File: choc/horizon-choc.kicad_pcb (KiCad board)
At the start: 2 copper layers, 252 x 68 mm, 63 parts, among them SW1 SW_Push, SW10 SW_Push, SW11 SW_Push, SW12 SW_Push, SW13 SW_Push, SW14 SW_Push, SW15 SW_Push, SW16 SW_Push, SW17 SW_Push, SW18 SW_Push, SW19 SW_Push, SW2 SW_Push, SW20 SW_Push, SW21 SW_Push, SW22 SW_Push, SW23 SW_Push, SW24 SW_Push, SW25 SW_Push, SW26 SW_Push, SW27 SW_Push, SW28 SW_Push, SW29 SW_Push, SW3 SW_Push, SW30 SW_Push, SW31 SW_Push, SW32 SW_Push, SW33 SW_Push, SW34 SW_Push, SW35 SW_Push, SW36 SW_Push, SW37 SW_Push, SW38 SW_Push, SW39 SW_Push, SW4 SW_Push, SW40 SW_Push, SW41 SW_Push, SW42 SW_Push, SW43 SW_Push, SW44 SW_Push, SW45 SW_Push, SW46 SW_Push, SW47 SW_Push, SW48 SW_Push, SW49 SW_Push, SW5 SW_Push, SW50 SW_Push, SW51 SW_Push, SW52 SW_Push, SW6 SW_Push, SW7 SW_Push, SW8 SW_Push, SW9 SW_Push, U1 PRO-MICRO

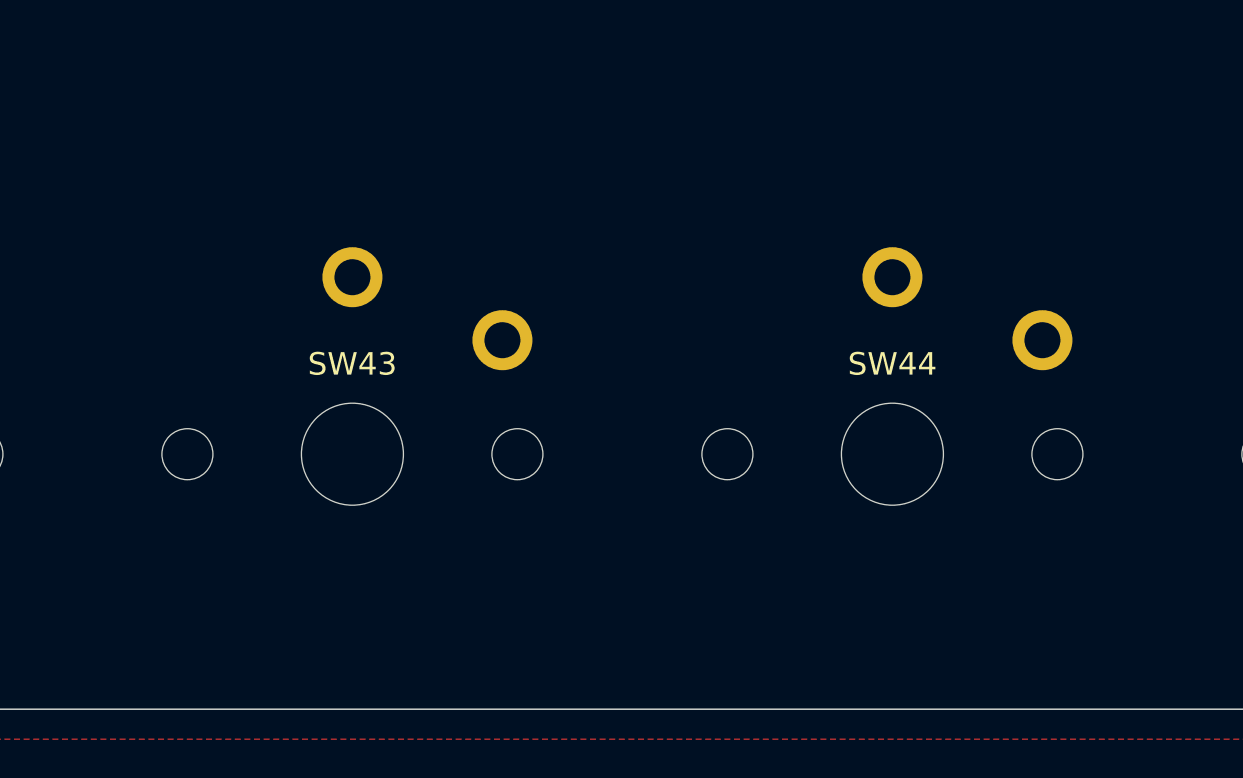
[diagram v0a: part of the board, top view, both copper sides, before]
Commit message: updated pcb
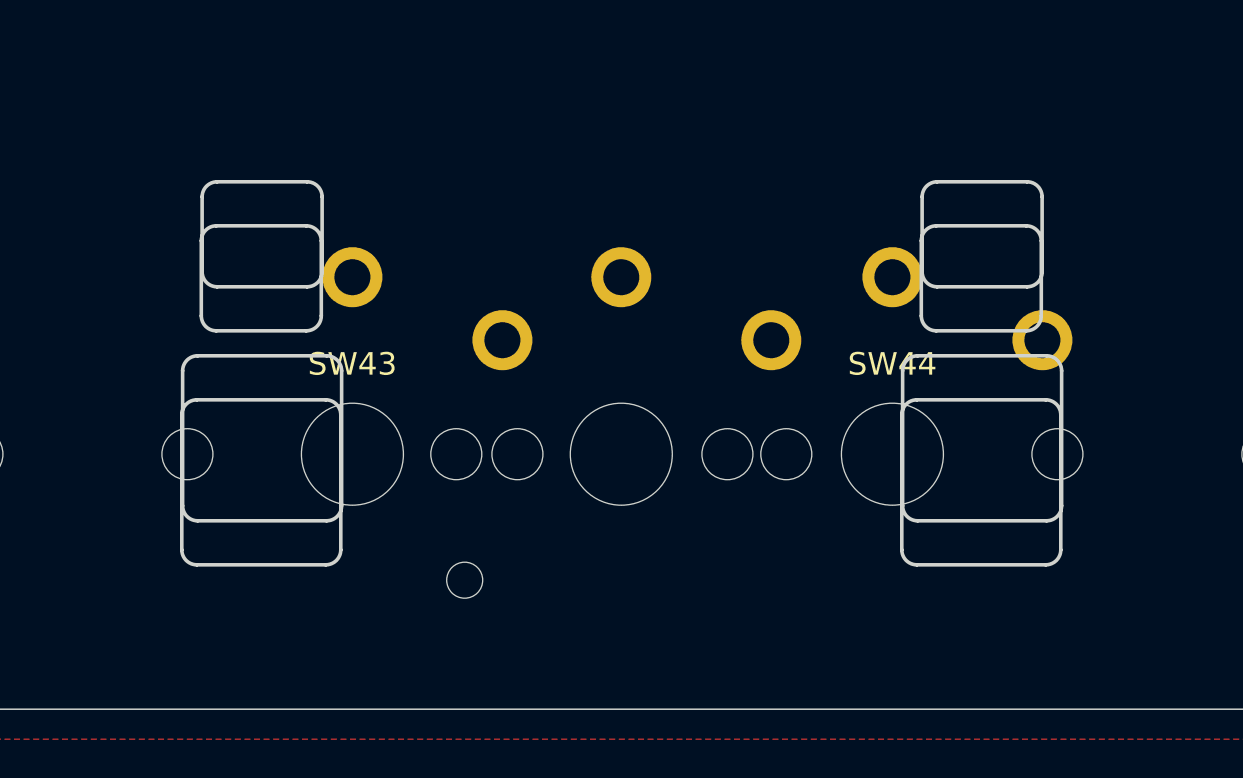
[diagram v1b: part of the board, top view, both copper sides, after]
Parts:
- added REF**: STAB_choc_2u, marbastlib-choc-untested:STAB_choc_2u, F.Cu at (112.0, 130.4)
- added REF**: STAB_choc_2u, marbastlib-choc-untested:STAB_choc_2u, F.Cu at (112.0, 131.9)
- added REF**: SW_choc_1u, marbastlib-choc:SW_choc_1u, F.Cu at (112.0, 130.5)
